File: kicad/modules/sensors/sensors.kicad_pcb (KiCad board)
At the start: 2 copper layers, 84.6 x 64 mm, 46 parts, among them J1 Bus_PCI_Express_x1, J2 TYPE-C-31-M-04, J4 Conn_01x02, U2 RP2040, U4 W25Q128JVP, U5 BMP388, U8 BNO055, U9 MCP25625T-E/ML, X1 ABM8-272-T3, Y1 ABS07-32.768KHZ-T, Y2 X322516MLB4SI

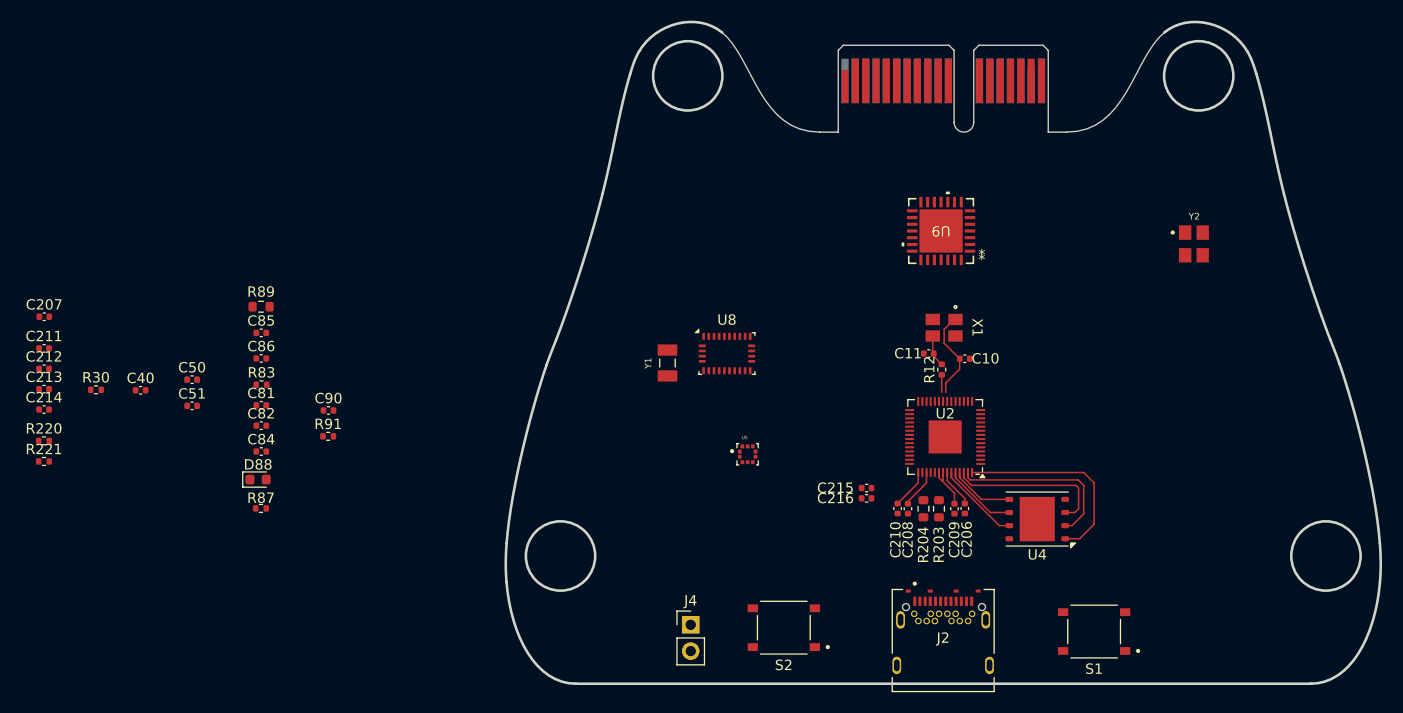
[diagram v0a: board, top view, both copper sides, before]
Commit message: continue routing
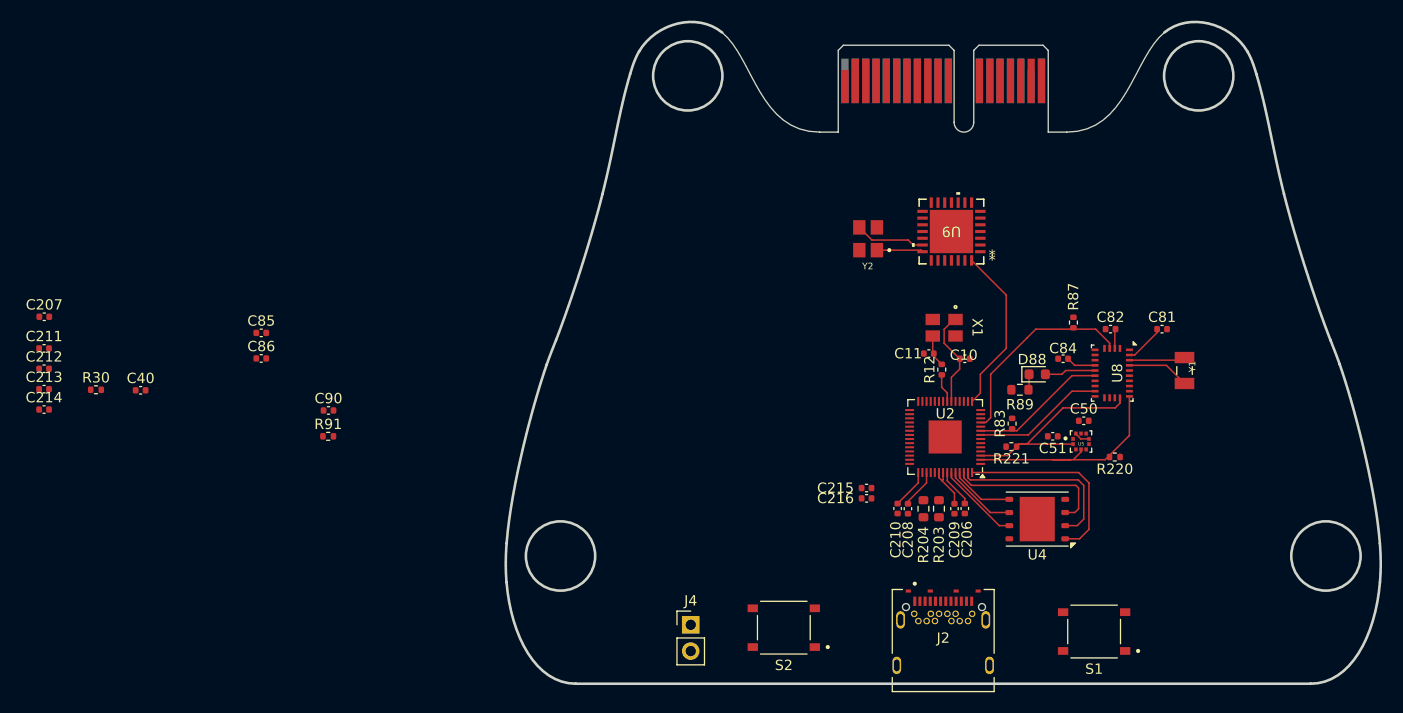
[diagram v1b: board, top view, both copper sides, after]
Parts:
- moved R220 103.5 mm to (163.0, 100.5), turned to 180 degrees
- moved R221 93.5 mm to (153.0, 99.5), turned to 180 degrees
- moved C81 87.4 mm to (167.6, 88.1)
- moved C50 86.3 mm to (160.0, 97.0)
- moved C51 83.3 mm to (157.0, 98.5), turned to 180 degrees
- moved C82 82.6 mm to (162.6, 88.1)
- moved R87 80.6 mm to (159.0, 87.5), turned to 90 degrees
- moved C84 78.0 mm to (158.0, 91.0)
- moved D88 76.0 mm to (155.5, 92.5)
- moved R89 73.8 mm to (153.8, 94.0), turned to 180 degrees
- moved R83 72.7 mm to (153.1, 97.3), turned to 90 degrees
- moved Y1 50.0 mm to (169.7, 92.1)
- moved U8 37.3 mm to (162.8, 92.4), turned to -90 degrees
- moved U5 32.3 mm to (159.7, 99.0)
- moved Y2 31.5 mm to (139.2, 79.4), turned to 180 degrees
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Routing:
- net SDA: track 0.00 -> 22.1 mm
- net SCL: track 0.00 -> 21.6 mm
- net BOOT_LOAD: track 0.00 -> 19.7 mm
- net SO: track 0.00 -> 16.4 mm
- net BNORESET: track 0.00 -> 13.3 mm
- net BNOINT: track 0.00 -> 12.8 mm
- net +3.3V: track 8.31 -> 15.6 mm
- net OSC2: track 0.00 -> 6.82 mm
- net Net-(U8-XOUT32): track 0.00 -> 6.05 mm
- net Net-(U8-XIN32): track 0.00 -> 5.43 mm
- net Net-(D88-A): track 0.00 -> 4.95 mm
- net OSC1: track 0.00 -> 4.47 mm
- net Net-(U8-CAP): track 0.00 -> 2.87 mm
- net Net-(D88-K): track 0.00 -> 1.53 mm
- net /XOUT: track 1.70 -> 2.79 mm
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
